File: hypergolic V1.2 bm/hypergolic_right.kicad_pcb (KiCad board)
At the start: 2 copper layers, 119.9 x 87.7 mm, 23 parts, among them SW10 SW_Push, SW11 SW_Push, SW12 SW_Push, SW14 SW_Push, SW15 SW_Push, SW16 SW_Push, SW17 SW_Push, SW18 SW_Push, SW2 SW_Push, SW20 SW_Push, SW21 SW_Push, SW3 SW_Push, SW4 SW_Push, SW5 SW_Push, SW6 SW_Push, SW8 SW_Push, SW9 SW_Push, U1 ProMicro-kbd

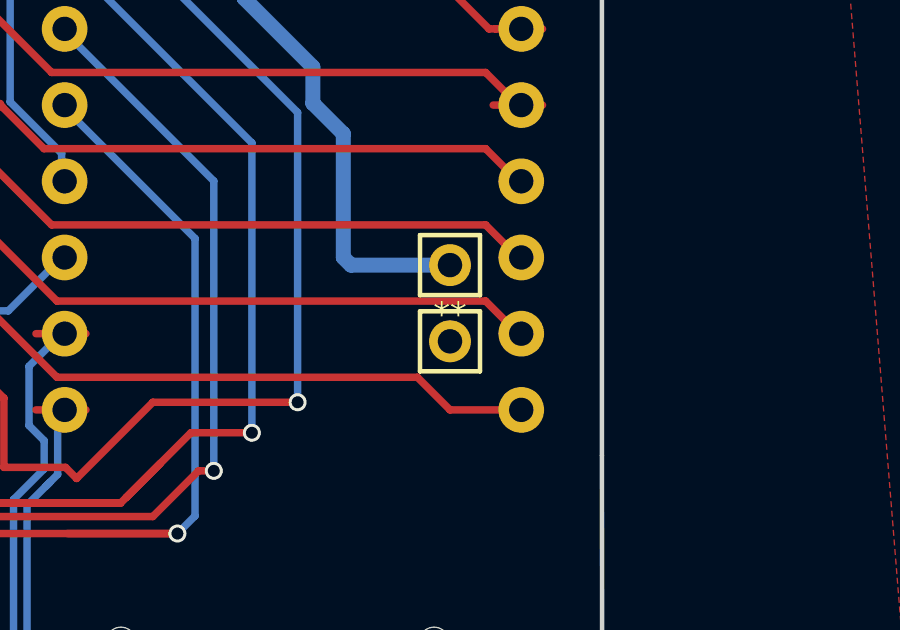
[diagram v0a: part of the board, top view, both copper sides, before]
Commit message: Add images for hypergolic 1.2bm
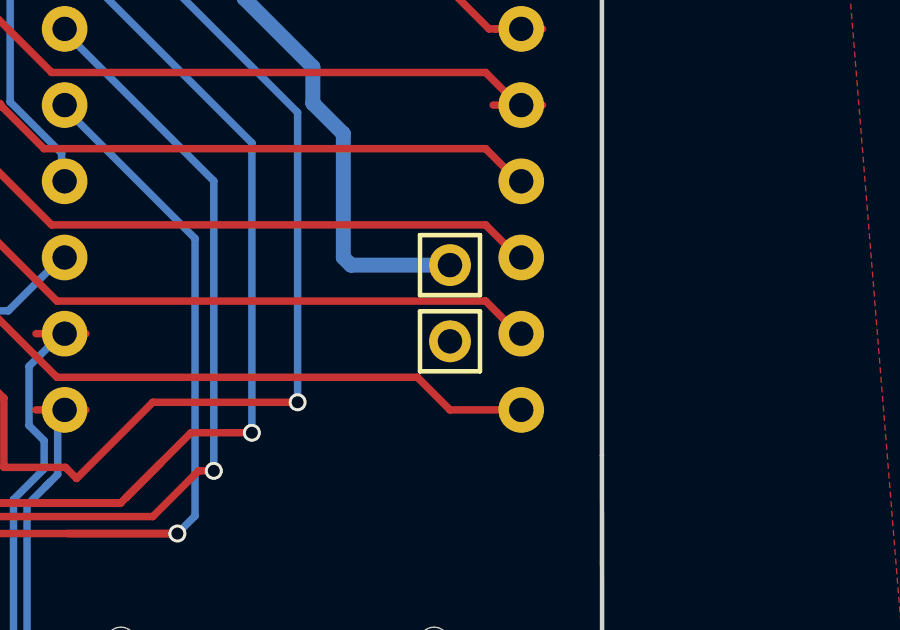
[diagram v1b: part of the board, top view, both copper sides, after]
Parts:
-  : renamed from **
